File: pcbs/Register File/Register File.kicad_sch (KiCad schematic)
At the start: 0 parts

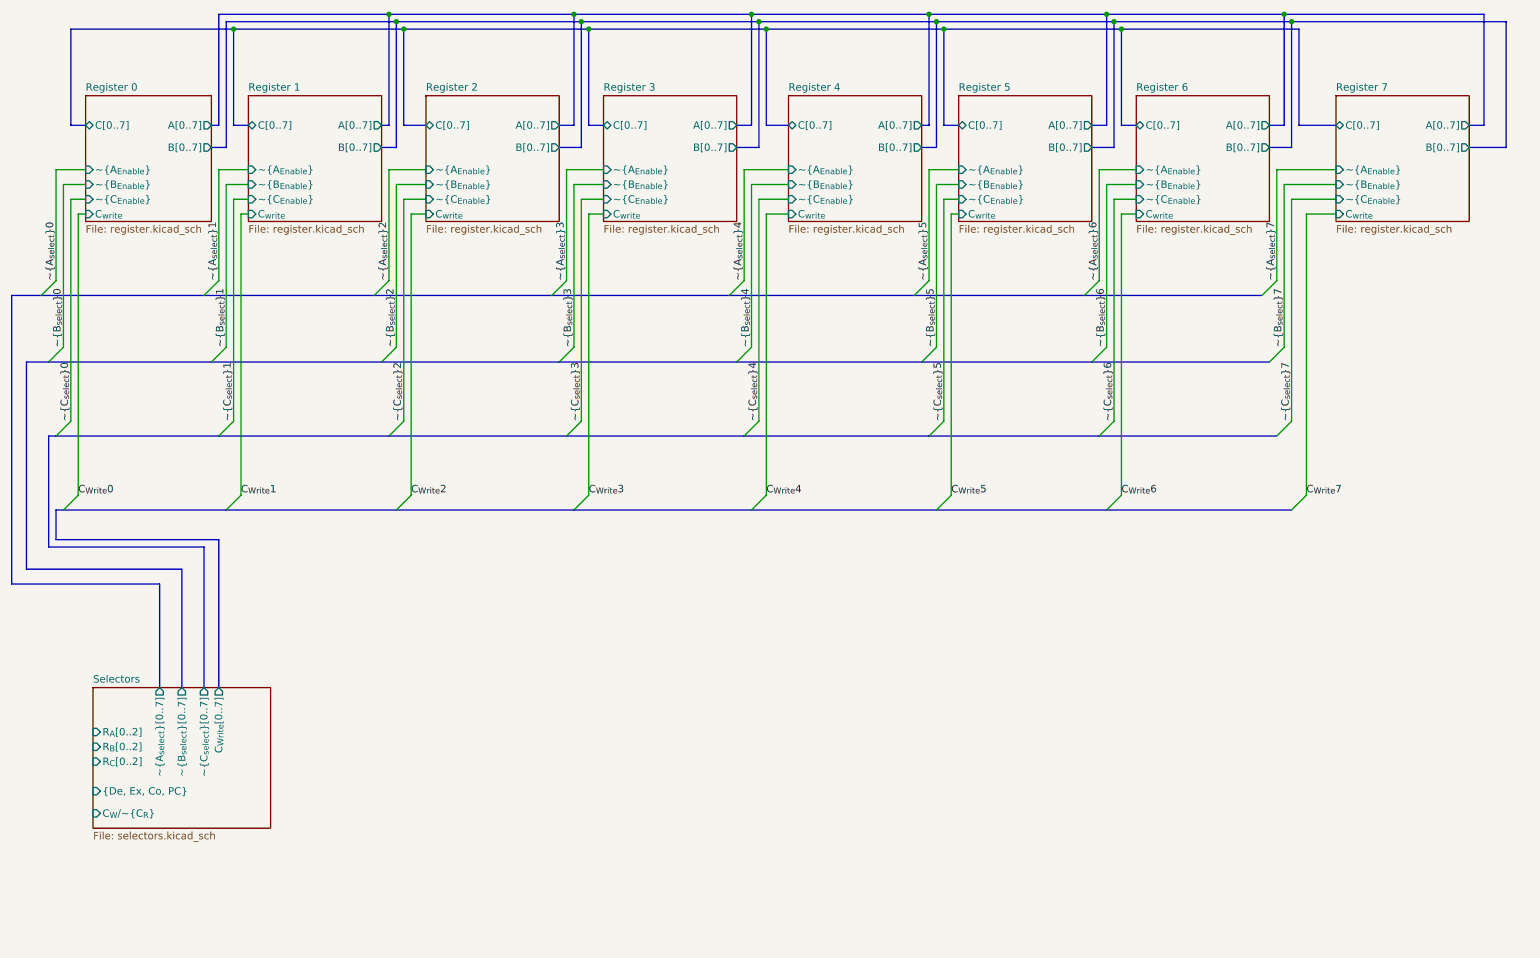
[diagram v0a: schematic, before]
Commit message: Routing the connector Pt 1 of n
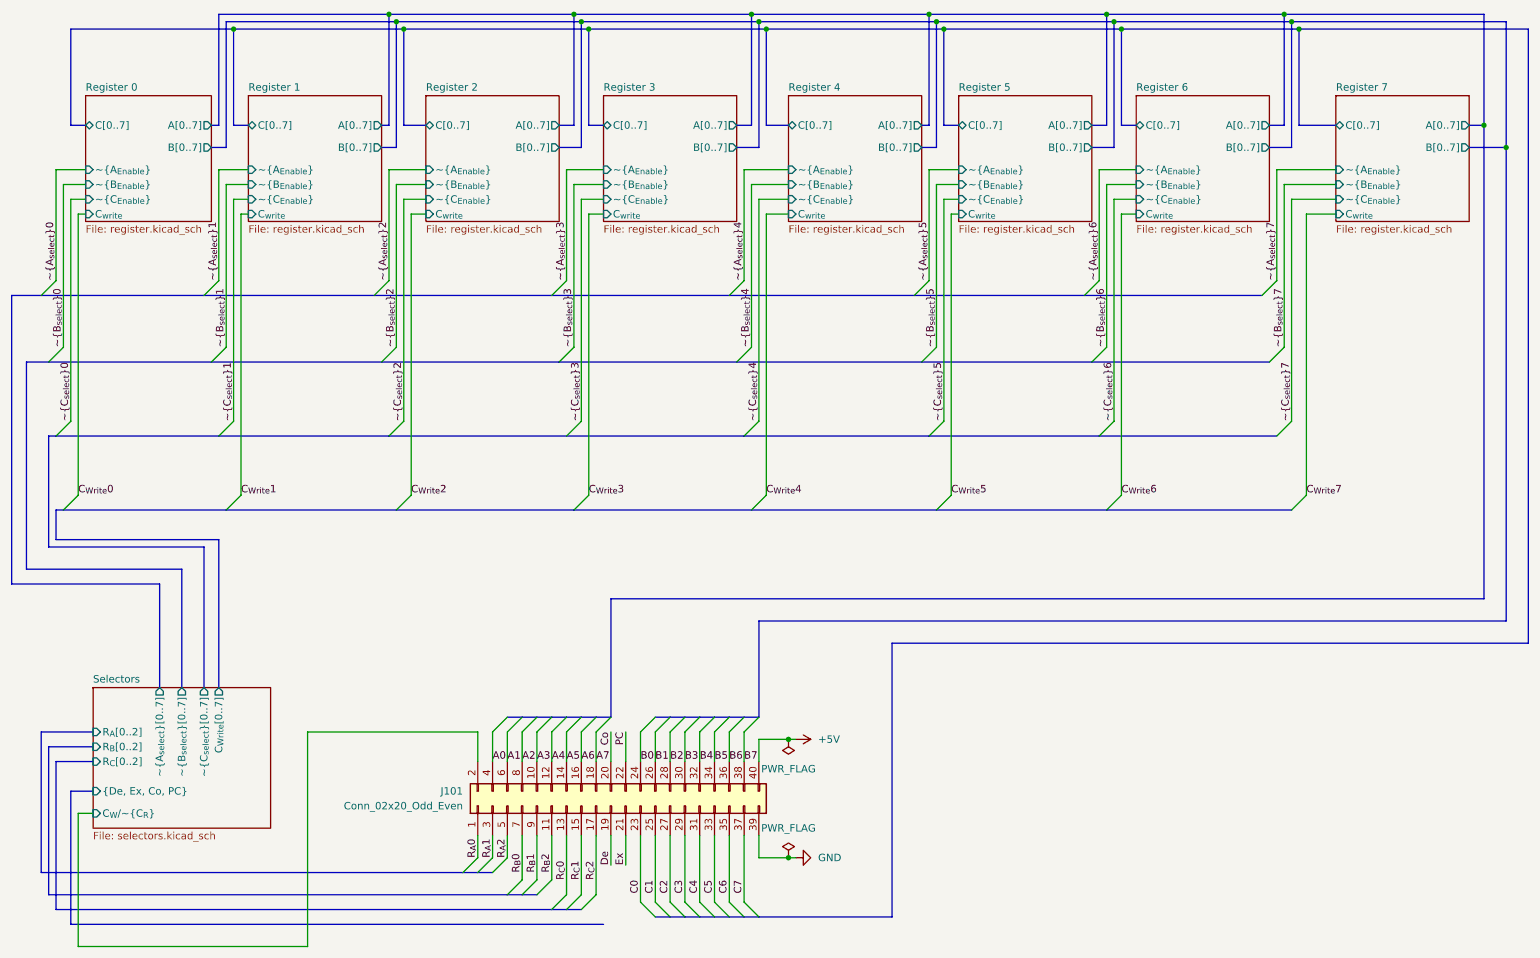
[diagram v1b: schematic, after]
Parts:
- added J101: Conn_02x20_Odd_Even, Connector_PinHeader_2.54mm:PinHeader_2x20_P2.54mm_Vertical, symbol Connector_Generic:Conn_02x20_Odd_Even
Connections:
- net Selectors/C_{W}/~{C_{R}}: now also J101.2 (Pin_2)
- new net +5V: J101.40 (Pin_40)
- new net A0: J101.4 (Pin_4)
- new net A1: J101.6 (Pin_6)
- new net A2: J101.8 (Pin_8)
- new net A3: J101.10 (Pin_10)
- new net A4: J101.12 (Pin_12)
- new net A5: J101.14 (Pin_14)
- new net A6: J101.16 (Pin_16)
- new net A7: J101.18 (Pin_18)
- new net B0: J101.24 (Pin_24)
- new net B1: J101.26 (Pin_26)
- new net B2: J101.28 (Pin_28)
- new net B3: J101.30 (Pin_30)
- new net B4: J101.32 (Pin_32)
- new net B5: J101.34 (Pin_34)
- new net B6: J101.36 (Pin_36)
- new net B7: J101.38 (Pin_38)
- new net C0: J101.23 (Pin_23)
- new net C1: J101.25 (Pin_25)
- new net C2: J101.27 (Pin_27)
- new net C3: J101.29 (Pin_29)
- new net C4: J101.31 (Pin_31)
- new net C5: J101.33 (Pin_33)
- new net C6: J101.35 (Pin_35)
- new net C7: J101.37 (Pin_37)
- new net Co: J101.20 (Pin_20)
- new net De: J101.19 (Pin_19)
- new net Ex: J101.21 (Pin_21)
- new net GND: J101.39 (Pin_39)
- new net PC: J101.22 (Pin_22)
- new net R_{A}0: J101.1 (Pin_1)
- new net R_{A}1: J101.3 (Pin_3)
- new net R_{A}2: J101.5 (Pin_5)
- new net R_{B}0: J101.7 (Pin_7)
- new net R_{B}1: J101.9 (Pin_9)
- new net R_{B}2: J101.11 (Pin_11)
- new net R_{C}0: J101.13 (Pin_13)
- new net R_{C}1: J101.15 (Pin_15)
- new net R_{C}2: J101.17 (Pin_17)
